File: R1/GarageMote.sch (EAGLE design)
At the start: 14 parts

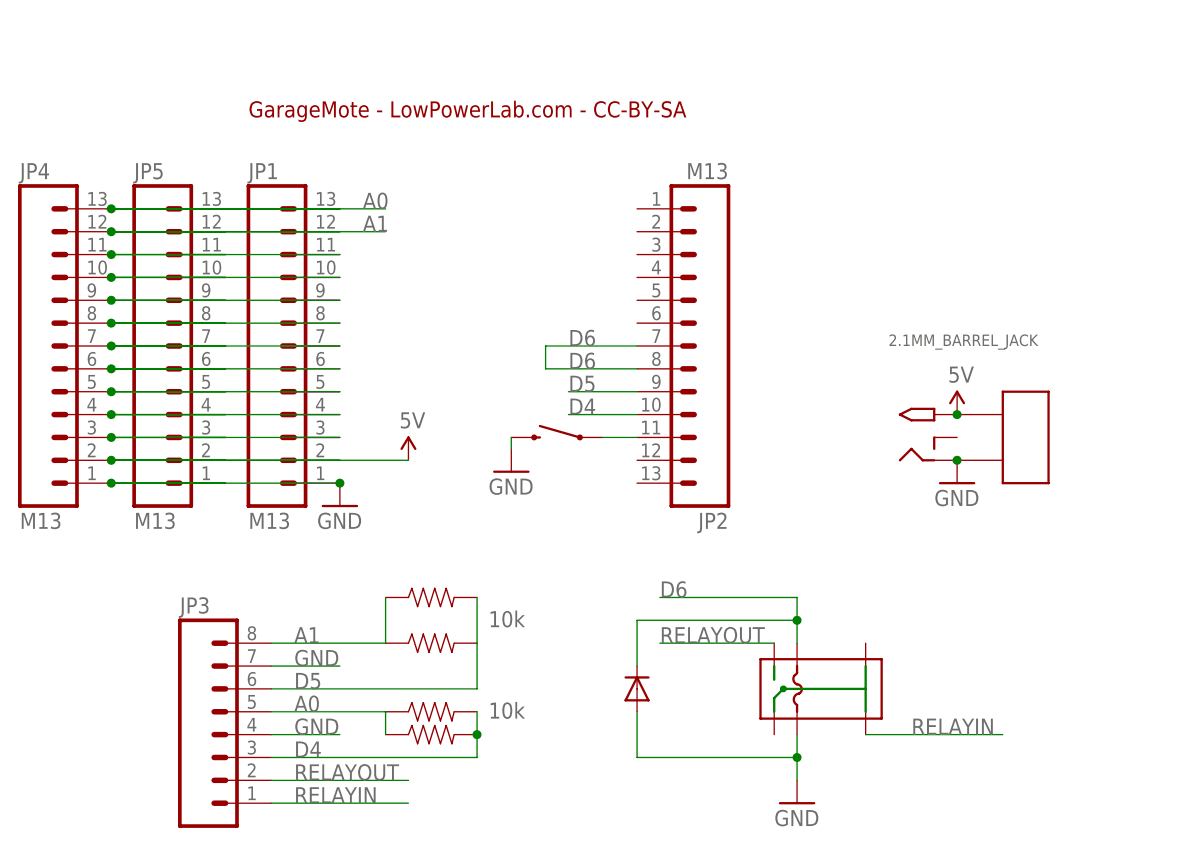
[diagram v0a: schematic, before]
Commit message: Add R2
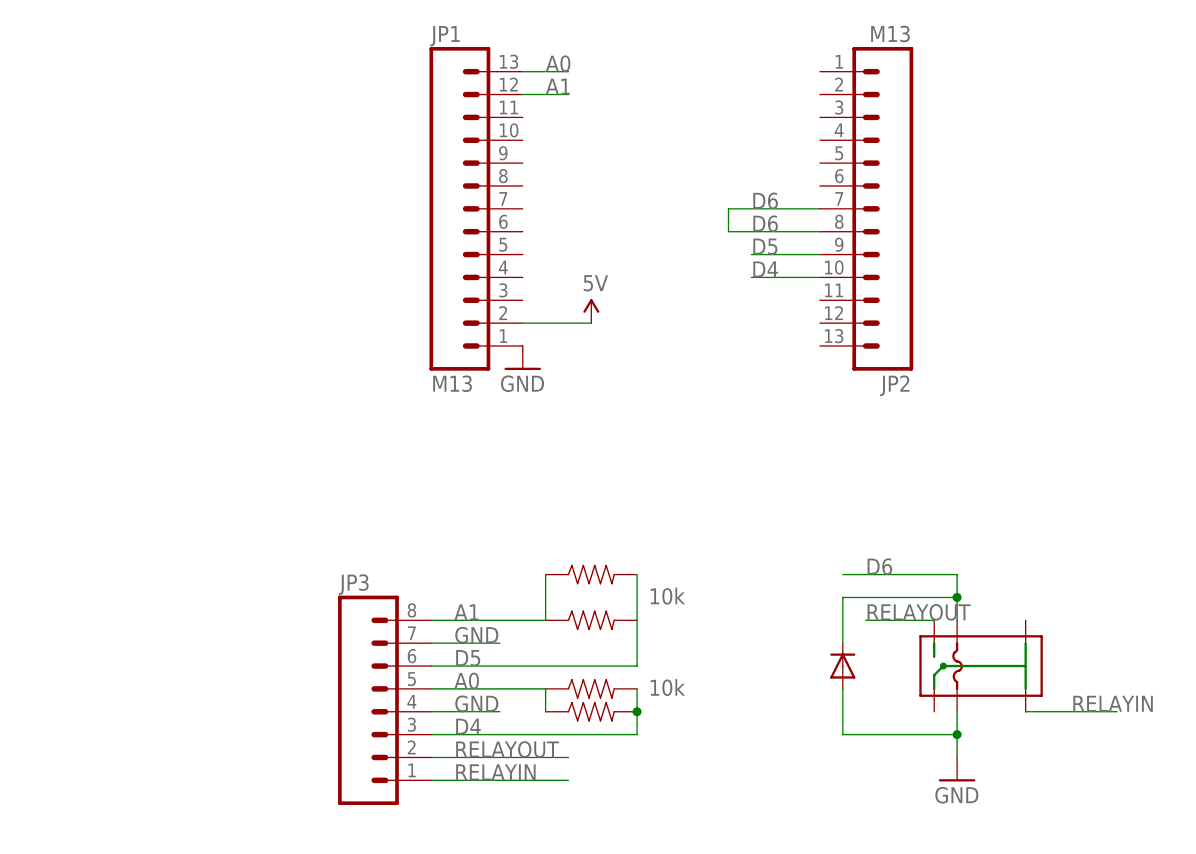
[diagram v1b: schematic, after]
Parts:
- removed 2.1MM_BARREL_JACK: 2.1MMJACKTH_NOSILK, LowPowerLab:2.1MMJACKTH_NOSILK
- removed JP4, JP5: M13, SparkFun-Connectors:M13
- removed S1: SWITCH-MOMENTARY-2SIDE_EZ, LowPowerLab:SWITCH-MOMENTARY-2SIDE_EZ
- removed U$4: DIODEPTH, LowPowerLab:DIODEPTH
- removed U$9: HDR_2PIN, LowPowerLab:HDR_2PIN
- added 1N4001: DIODEUPRIGHT, LowPowerLab:DIODEUPRIGHT
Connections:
- removed net N$1: JP2.11, S1.1
- removed net N$10: JP1.11, JP4.11, JP5.11
- removed net N$2: JP1.3, JP4.3, JP5.3
- removed net N$3: JP1.4, JP4.4, JP5.4
- removed net N$4: JP1.5, JP4.5, JP5.5
- removed net N$5: JP1.6, JP4.6, JP5.6
- removed net N$6: JP1.7, JP4.7, JP5.7
- removed net N$7: JP1.8, JP4.8, JP5.8
- removed net N$8: JP1.9, JP4.9, JP5.9
- removed net N$9: JP1.10, JP4.10, JP5.10
- net 5V: no longer 2.1MM_BARREL_JACK.TIP, JP4.2, JP5.2, U$9.P$1
- net A0: no longer JP4.13, JP5.13
- net A1: no longer JP4.12, JP5.12
- net D6: now also 1N4001.CATHODE_MINUS; no longer U$4.CATHODE_MINUS
- net GND: now also 1N4001.ANODE_PLUS; no longer 2.1MM_BARREL_JACK.RING, JP4.1, JP5.1, S1.2, U$4.ANODE_PLUS, U$9.P$2
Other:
- note removed: "GarageMote - LowPowerLab.com - CC-BY-SA"
- moved on the sheet: JP1, JP2, JP3
